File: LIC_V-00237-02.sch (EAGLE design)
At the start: 17 parts, among them J1 S4B-PH-SM4-TB

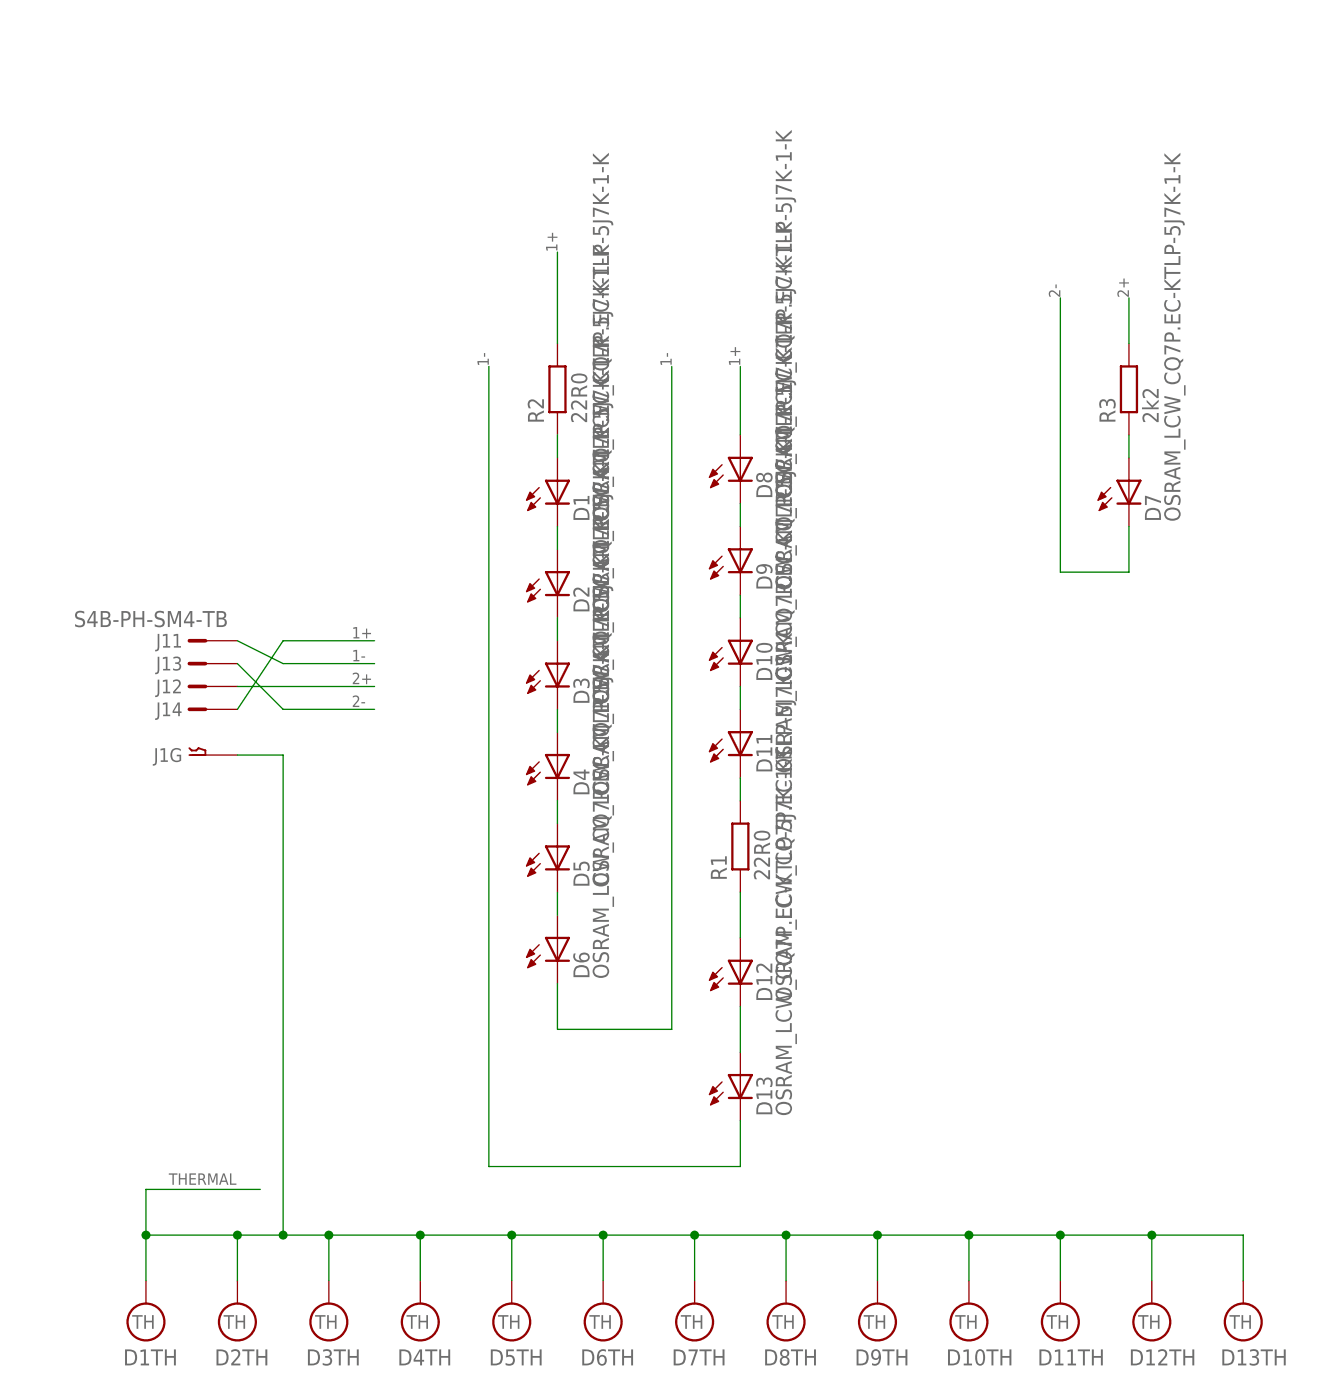
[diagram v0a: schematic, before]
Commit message: Další verze
Verze pro normální LED
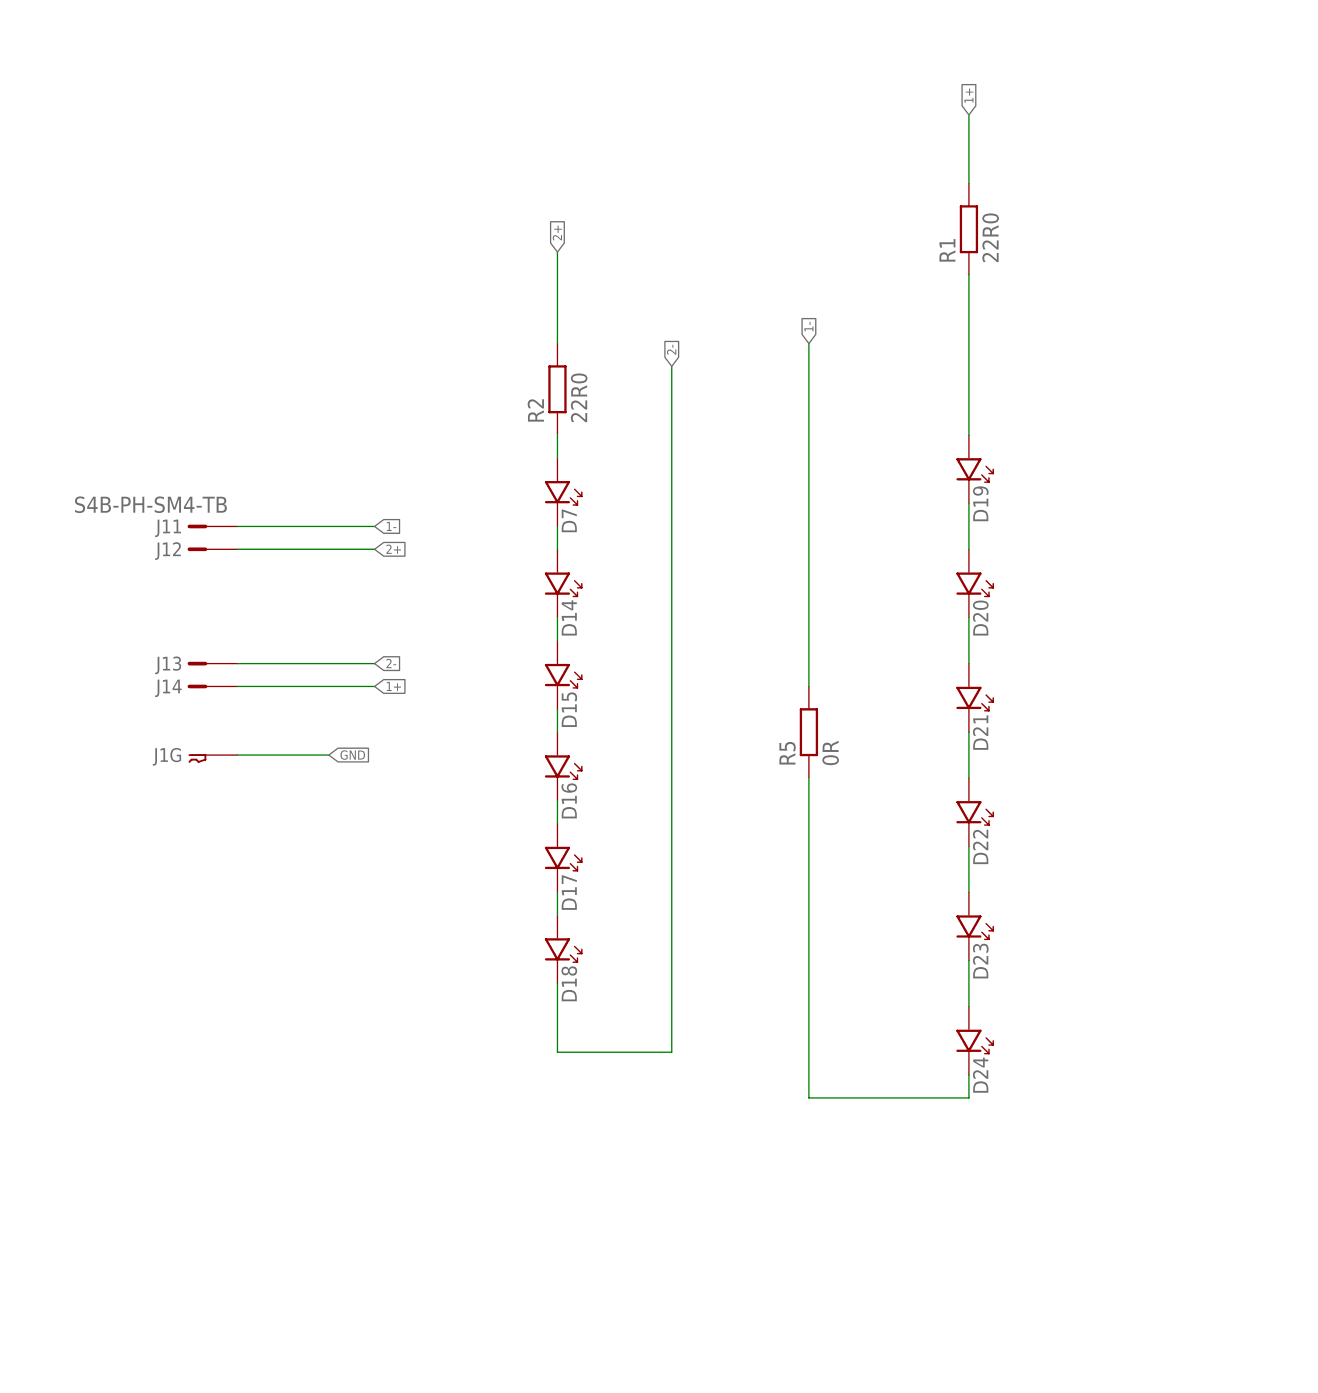
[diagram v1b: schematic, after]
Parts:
- removed D1, D10, D11, D12, D13, D2, D3, D4, D5, D6, D8, D9: OSRAM_LCW_CQ7P.EC-KTLP-5J7K-1-K, led:OSRAM_LCW_CQ7P.EC-KTLP-5J7K-1-K
- removed R3: 2k2, rcl:R-EU_R1206
- added D14, D15, D16, D17, D18, D19, D20, D21, D22, D23, D24: (no value), #PaJa_31:LED_1206
- added R5: 0R, rcl:R-EU_R1206
- D7: value OSRAM_LCW_CQ7P.EC-KTLP-5J7K-1-K -> (none); device led:OSRAM_LCW_CQ7P.EC-KTLP-5J7K-1-K -> #PaJa_31:LED_1206
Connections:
- removed net THERMAL: D10TH.TH, D11TH.TH, D12TH.TH, D13TH.TH, D1TH.TH, D2TH.TH, D3TH.TH, D4TH.TH, D5TH.TH, D6TH.TH, D7TH.TH, D8TH.TH, D9TH.TH, J1G.1
- new net GND: J1G.1
- net 1+: now also R1.2; no longer D8LED.A, R2.2
- net 1-: now also R5.2; no longer D13LED.C, D6LED.C
- net 2+: now also R2.2; no longer R3.2
- net 2-: now also D18.K; no longer D7LED.C
- net N$1: now also D14.A, D7.K; no longer D1LED.C, D2LED.A
- net N$10: now also D22.K, D23.A; no longer D12LED.A, R1.1
- net N$11: now also D19.A, R1.1; no longer D11LED.C, R1.2
- net N$12: now also D24.K, R5.1; no longer D7LED.A, R3.1
- net N$14: now also D23.K, D24.A; no longer D12LED.C, D13LED.A
- net N$2: now also D14.K, D15.A; no longer D2LED.C, D3LED.A
- net N$3: now also D15.K, D16.A; no longer D3LED.C, D4LED.A
- net N$4: now also D16.K, D17.A; no longer D4LED.C, D5LED.A
- net N$5: now also D17.K, D18.A; no longer D5LED.C, D6LED.A
- net N$6: now also D7.A; no longer D1LED.A
- net N$7: now also D19.K, D20.A; no longer D8LED.C, D9LED.A
- net N$8: now also D20.K, D21.A; no longer D10LED.A, D9LED.C
- net N$9: now also D21.K, D22.A; no longer D10LED.C, D11LED.A
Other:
- moved on the sheet: J11, J12, J14, J1G, R1
